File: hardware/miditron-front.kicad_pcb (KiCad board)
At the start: 2 copper layers, 39.4 x 109.2 mm, 34 parts, among them J10 PJ398SM, J11 PJ398SM, J12 PJ398SM, J13 PJ398SM, J14 PJ398SM, J15 PJ398SM, J16 PJ398SM, J17 PJ398SM, J18 PJ398SM, J19 PJ398SM, J20 PJ398SM, J21 PJ398SM, J22 PJ398SM, J23 PJ398SM, J24 PJ398SM, J25 PJ398SM, J26 PJ398SM, J27 PJ398SM, J28 PJ398SM, J29 PJ398SM, J30 PJ398SM, J31 PJ398SM, J5 Conn_02x06_Odd_Even, J6 Conn_02x06_Odd_Even, J7 Conn_01x10, J8 Conn_01x12, J9 SD-50BV

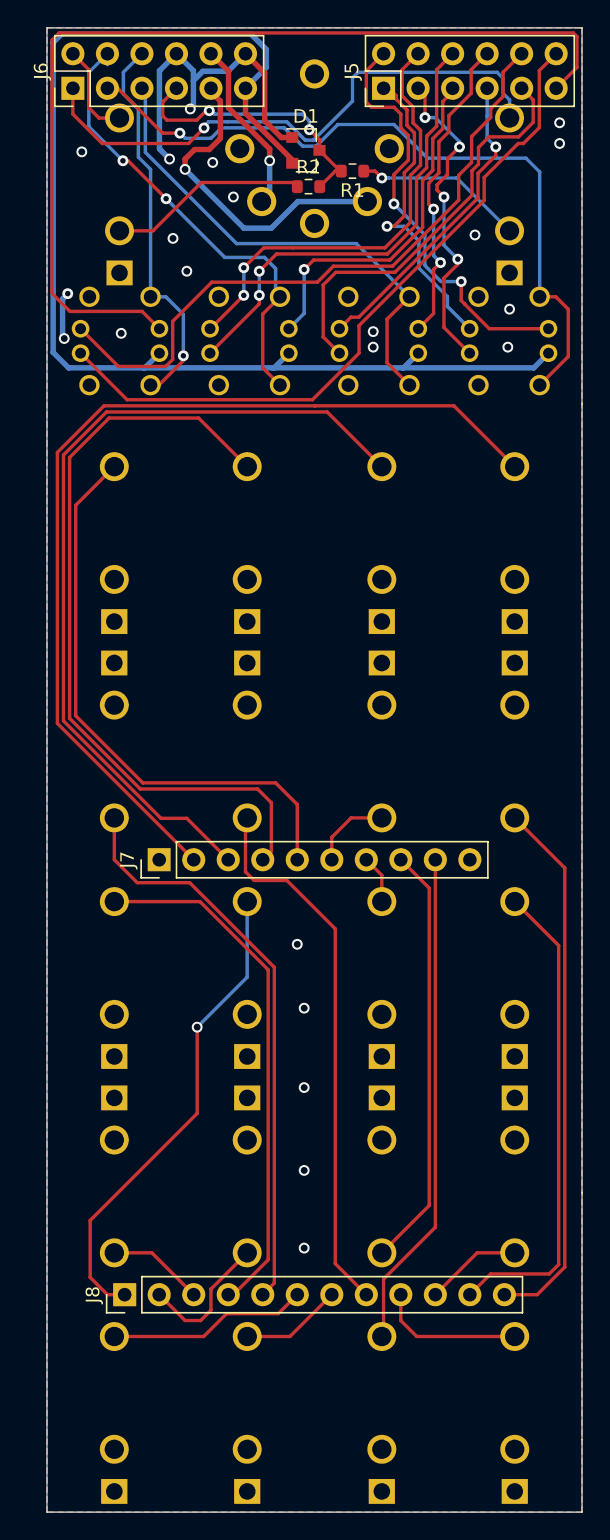
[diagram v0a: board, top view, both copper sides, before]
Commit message: split up pcb into two projects
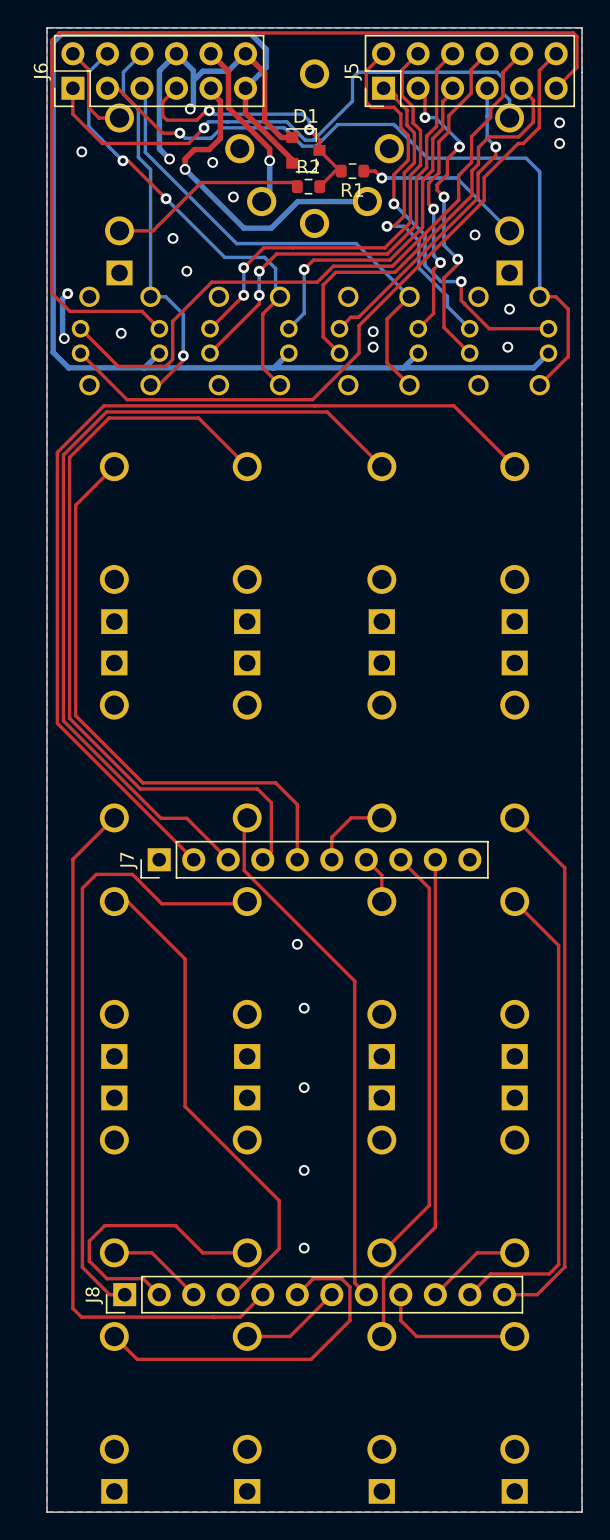
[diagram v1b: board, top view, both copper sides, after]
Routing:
- net dac8_out_h_front: track 14.7 -> 26.3 mm
- net dac8_out_e_front: track 10.2 -> 20.6 mm
- net dac8_out_c_front: track 35.5 -> 45.4 mm, vias 1 -> 0
- net dac8_out_b_front: track 42.6 -> 52.3 mm
- net dac8_out_d_front: track 38.7 -> 36.3 mm
- net dac8_out_a_front: track 40.2 -> 38.9 mm
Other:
- outline, holes or cut-outs redrawn
